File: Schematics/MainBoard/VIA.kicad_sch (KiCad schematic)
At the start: 6 parts, among them IC3 W65C22S6TQG-14, J11 Conn_02x04_Odd_Even, J12 Conn_02x06_Odd_Even, J13 Conn_02x06_Odd_Even

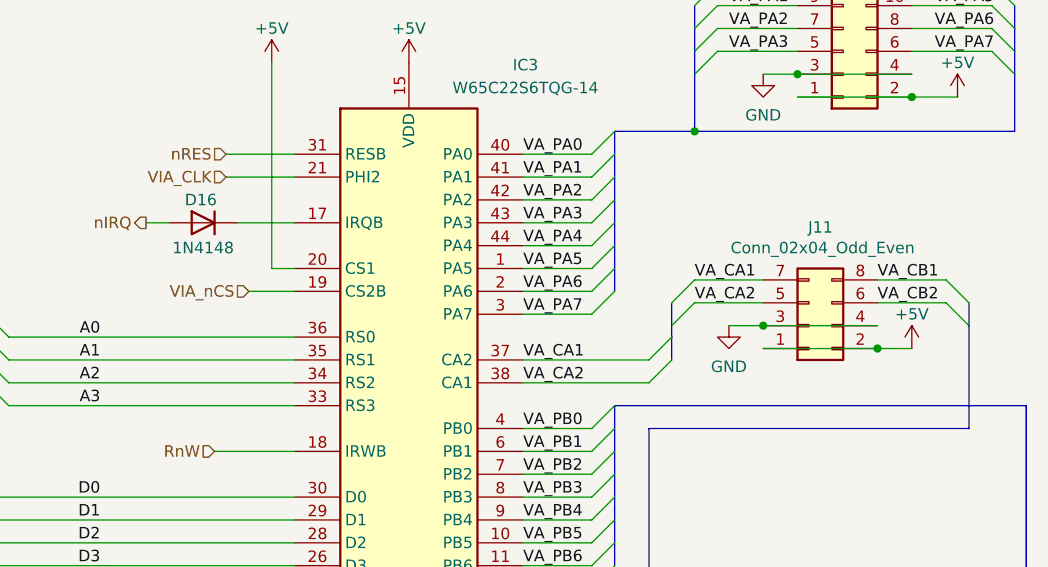
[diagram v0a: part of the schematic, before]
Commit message: Work on PCB
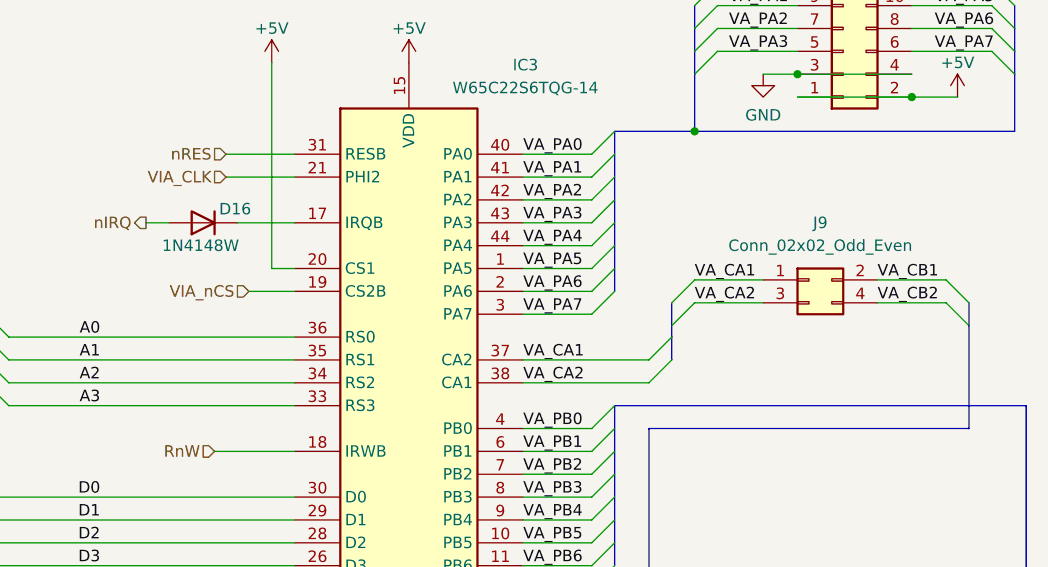
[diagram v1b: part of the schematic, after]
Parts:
- removed D16: 1N4148, Diode_THT:D_DO-35_SOD27_P7.62mm_Horizontal, symbol Diode:1N4148
- removed J11: Conn_02x04_Odd_Even, Connector_PinSocket_2.54mm:PinSocket_2x04_P2.54mm_Horizontal, symbol Connector_Generic:Conn_02x04_Odd_Even
- added D16: 1N4148W, Diode_SMD:D_SOD-123, symbol Diode:1N4148W
- added J9: Conn_02x02_Odd_Even, Connector_PinHeader_1.27mm:PinHeader_2x02_P1.27mm_Vertical_SMD, symbol Connector_Generic:Conn_02x02_Odd_Even
- C47: footprint Capacitor_SMD:C_0603_1608Metric -> Capacitor_SMD:C_0402_1005Metric
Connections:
- net VA_CA1: now also J9.1 (Pin_1)
- net VA_CA2: now also J9.3 (Pin_3)
- net VA_CB1: now also J9.2 (Pin_2)
- net VA_CB2: now also J9.4 (Pin_4)
- net nIRQ: now also D16.2 (A)
- net at IC3.17 (IRQB): now also D16.1 (K)
